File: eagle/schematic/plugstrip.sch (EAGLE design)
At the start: 20 parts, among them U1 Hall Effect, U2 Current ADC, U3 Voltage ADC

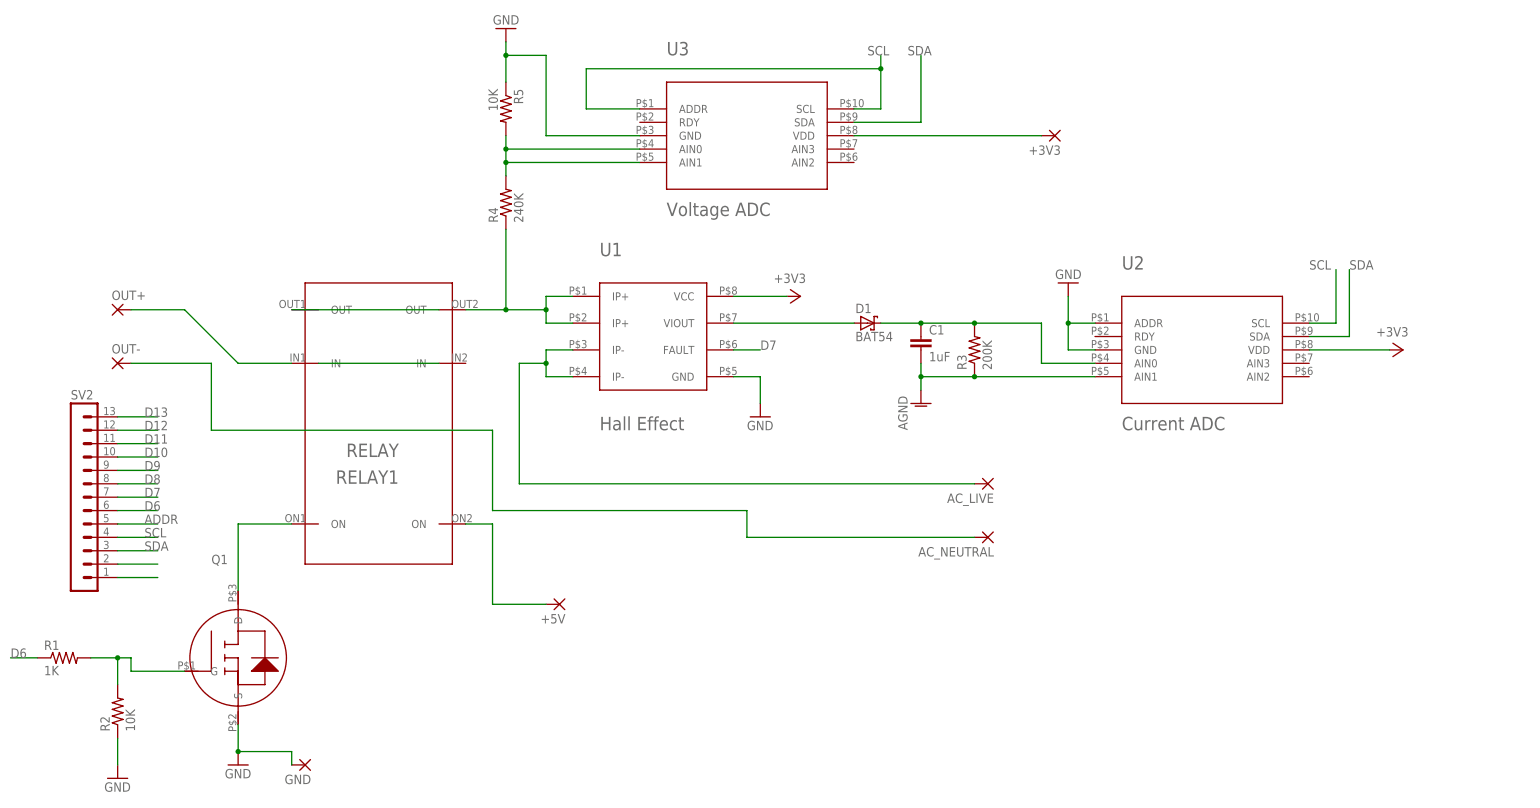
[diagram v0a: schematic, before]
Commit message: more schematic?
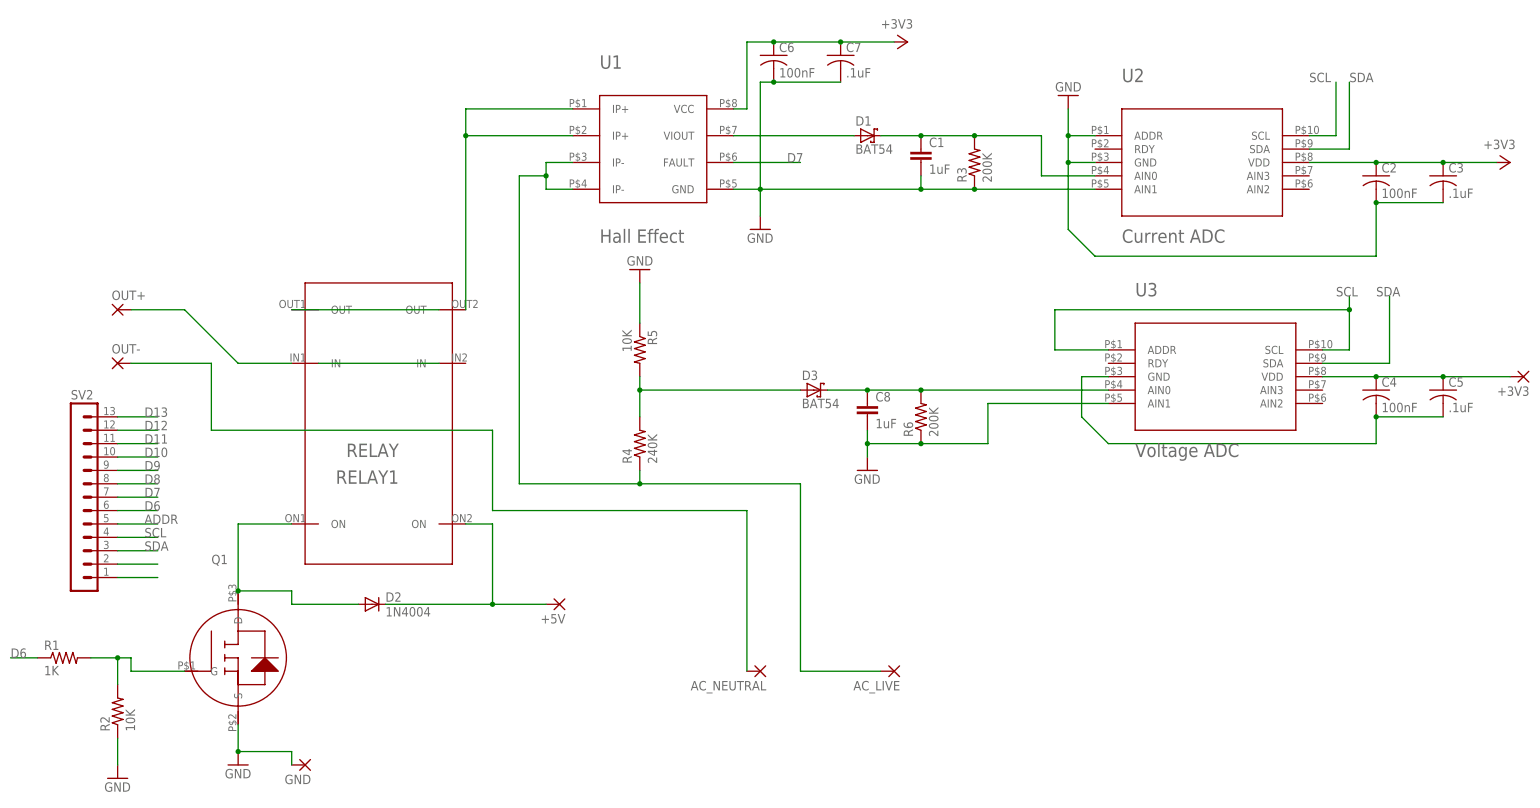
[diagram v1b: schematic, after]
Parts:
- added C2, C4, C6: 100nF, rcl:C-USC1206
- added C3, C5, C7: .1uF, rcl:C-USC1206
- added C8: 1uF, jackIdd:CSR215E105
- added D2: 1N4004, diode:1N4004
- added D3: BAT54, diode:BAT54
- added R6: 200K, jackIdd:R-US_CT14J
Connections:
- removed net AGND: C1.2, R3.1, U2.AIN1
- removed net N$5 (its old number): Q1.D, RELAY1.ON@1
- new net N$13: RELAY1.OUT@2, U1.IP+@1, U1.IP+@2
- new net N$14: C4.2, C5.2, U3.GND
- new net N$15: C8.1, D3.C, R6.2, U3.AIN0
- net +3V3: now also C2.1, C3.1, C6.1, C7.1
- net AC_LIVE: now also R4.1
- net GND: now also C1.2, C2.2, C3.2, C6.2, C7.2, C8.2, R3.1, R6.1, U2.AIN1, U3.AIN1; no longer U3.GND
- net N$12: now also D2.C
- net N$3: now also +3V3.P, C4.1, C5.1, U3.VDD; no longer R4.1, RELAY1.OUT@2, U1.IP+@1, U1.IP+@2
- net N$31: now also D3.A; no longer U3.AIN0, U3.AIN1
- net N$4: now also D2.A, Q1.D, RELAY1.ON@1; no longer +3V3.P, U3.VDD
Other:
- moved on the sheet: +3V3, AC_LIVE, AC_NEUTRAL, C1, D1, R3, R4, R5, U1, U2, U3
